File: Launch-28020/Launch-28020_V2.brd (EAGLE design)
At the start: 74.1 x 48 mm, 26 parts, among them X1 C-GRID-06-74099, X2 C-GRID-04-74099, X3 C-GRID-06-74099, X4 C-GRID-08-74099, X5 C-GRID-07-74099, X6 C-GRID-03-74099, X7 C-GRID-03-74099, X8 C-GRID-03-74099, X9 C-GRID-03-74099

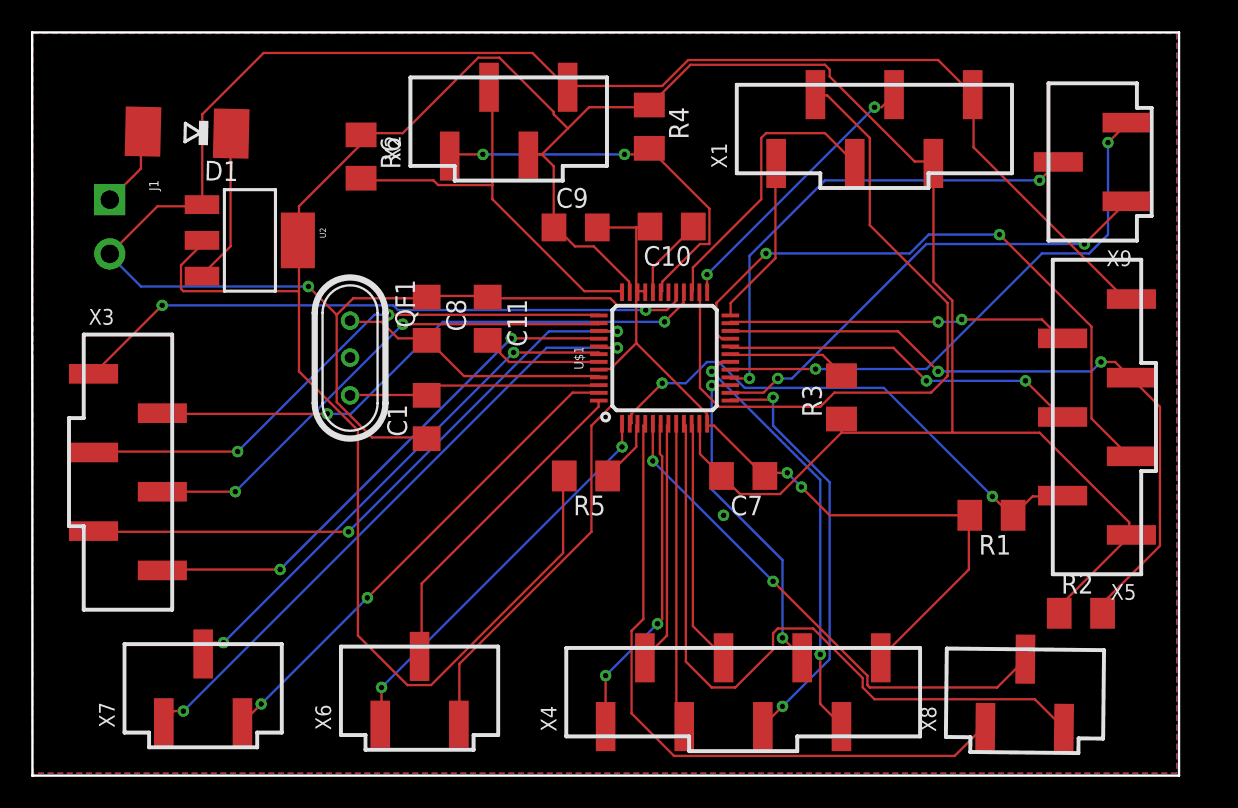
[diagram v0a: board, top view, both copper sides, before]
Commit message: Updated Layout
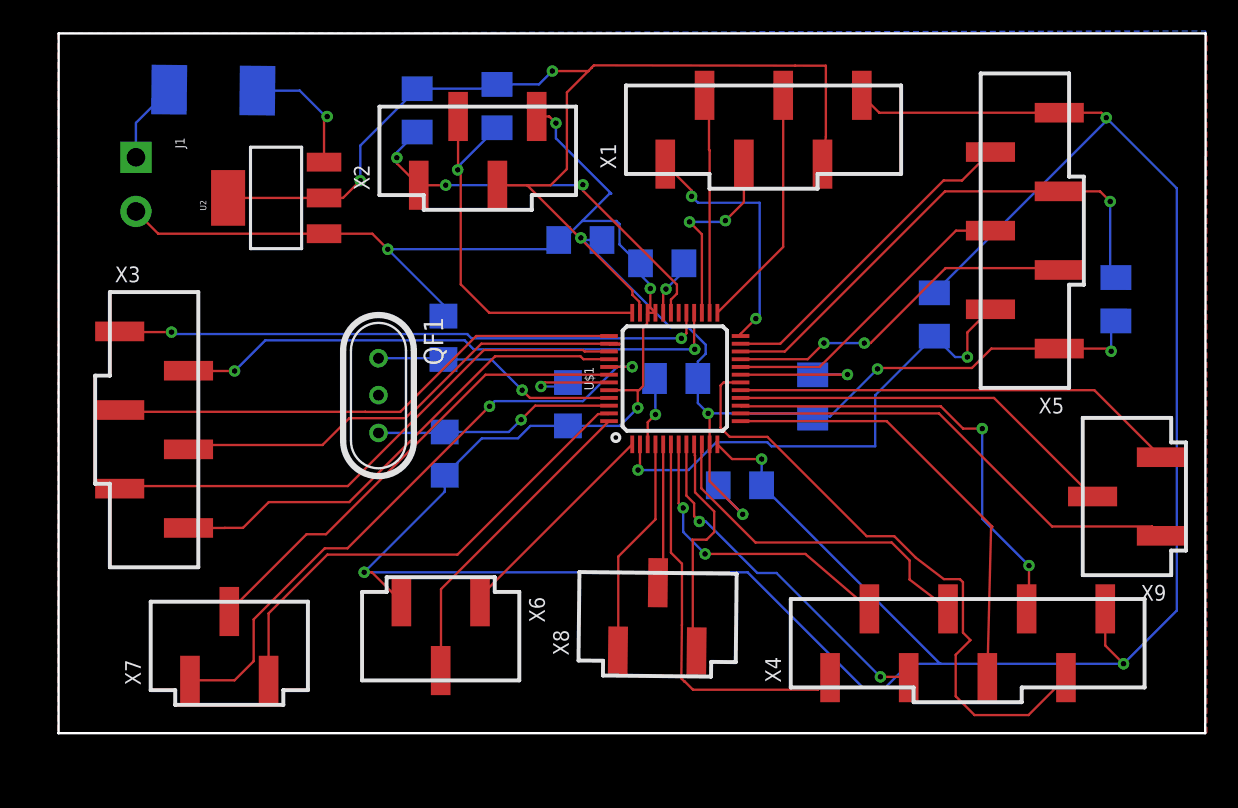
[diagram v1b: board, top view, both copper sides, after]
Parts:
- moved X8 24.2 mm to (41.5, 16.3)
- moved X9 21.7 mm to (71.8, 24.1)
- moved R2 20.4 mm to (71.1, 36.8), flipped to the bottom, turned to 90.1 degrees
- moved R4 15.0 mm to (25.9, 49.0), flipped to the bottom
- moved X4 14.8 mm to (61.5, 14.6)
- moved R1 13.5 mm to (59.3, 35.8), flipped to the bottom, turned to 90 degrees
- moved X5 12.9 mm to (65.2, 41.2)
- moved R6 9.37 mm to (31.1, 49.3), flipped to the bottom
- moved R5 8.58 mm to (42.7, 31.7), flipped to the bottom
- moved C11 7.58 mm to (35.7, 30.0), flipped to the bottom, turned to 90 degrees
- moved X1 7.16 mm to (48.3, 47.8)
- moved X6 3.79 mm to (27.4, 15.0), turned to 180 degrees
- moved X3 3.22 mm to (8.93, 28.4)
- moved D1 3.22 mm to (12.8, 50.3), flipped to the bottom, turned to 0.6 degrees
- moved U2 3.22 mm to (16.8, 43.4), turned to 90 degrees
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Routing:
- net VDD: track 192.7 -> 130.5 mm, vias 0 -> 7
- net SPI_MISO: track 45.7 -> 14.2 mm
- net AIO2: track 45.8 -> 15.4 mm
- net AIO6: track 43.8 -> 14.4 mm
- net GND: track 214.1 -> 239.9 mm, vias 3 -> 8
- net AIO4: track 33.7 -> 9.08 mm, vias 2 -> 0
- net TMS: track 41.1 -> 23.1 mm
- net ADC_B7: track 27.9 -> 40.4 mm, vias 2 -> 0
- net UART_TX: track 26.0 -> 14.2 mm, vias 2 -> 0
- net TDO: track 45.2 -> 33.6 mm, vias 2 -> 1
- net ADC_B3: track 21.2 -> 29.2 mm
- net AIO14: track 35.8 -> 29.0 mm, vias 2 -> 0
- net ADC_A0: track 16.0 -> 22.6 mm
- net AIO12: track 31.7 -> 25.4 mm, vias 2 -> 0
- net SPI_MOSI: track 18.8 -> 12.7 mm, vias 0 -> 2
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- added copper zone on layer 1, net N$2
- added copper zone on layer 16, net S$1
- removed copper zone on layer 16, net N$11
- removed copper zone on layer 1, net N$13
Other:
- board size 74.1 x 48 mm -> 74.1 x 45.2 mm
